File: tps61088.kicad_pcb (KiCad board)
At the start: 2 copper layers, 102 x 101.8 mm, 114 parts, among them J10 Conn_01x04, J11 Conn_01x04, J12 Conn_01x04, J13 Conn_01x04, J14 Conn_01x04, J2 Conn_01x12, J3 Conn_01x08, J5 Conn_01x02, J6 Conn_01x02, J7 Conn_01x04, J8 Conn_01x04, J9 Conn_01x04, P1 USB_C_Plug_USB2.0, SW1 SW_SPDT, SW2 SW_SPDT, SW3 SW_SPDT, SW4 SW_SPDT, SW5 SW_SPDT, SW6 SW_SPDT, SW7 SW_SPDT, U1 tps61088, U2 TPS5430DDA, U3 TPS5430DDA, U4 TPS5430DDA, U5 TPS5430DDA

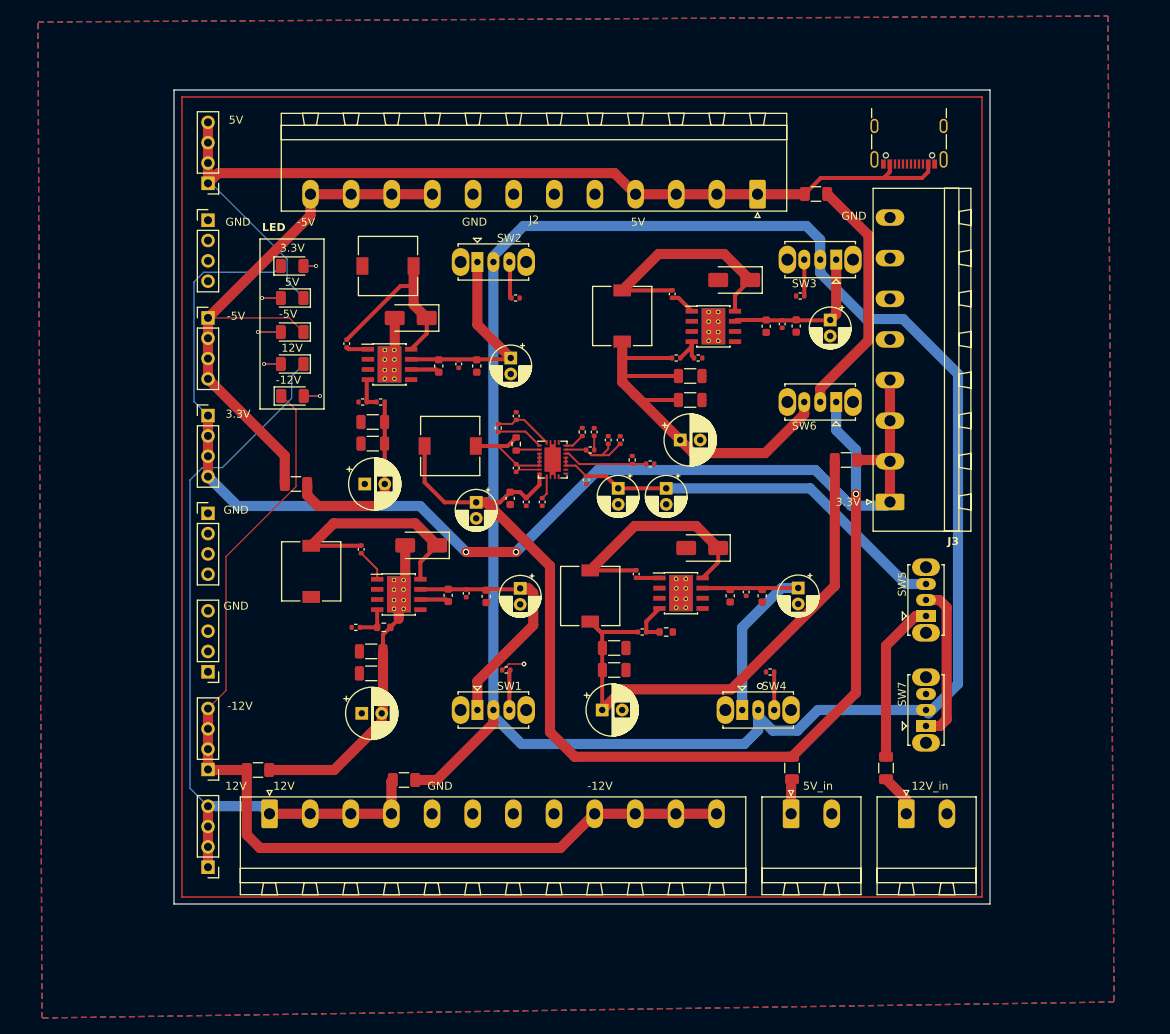
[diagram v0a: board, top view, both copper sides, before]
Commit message: V1.0
第一次下单PCB文件
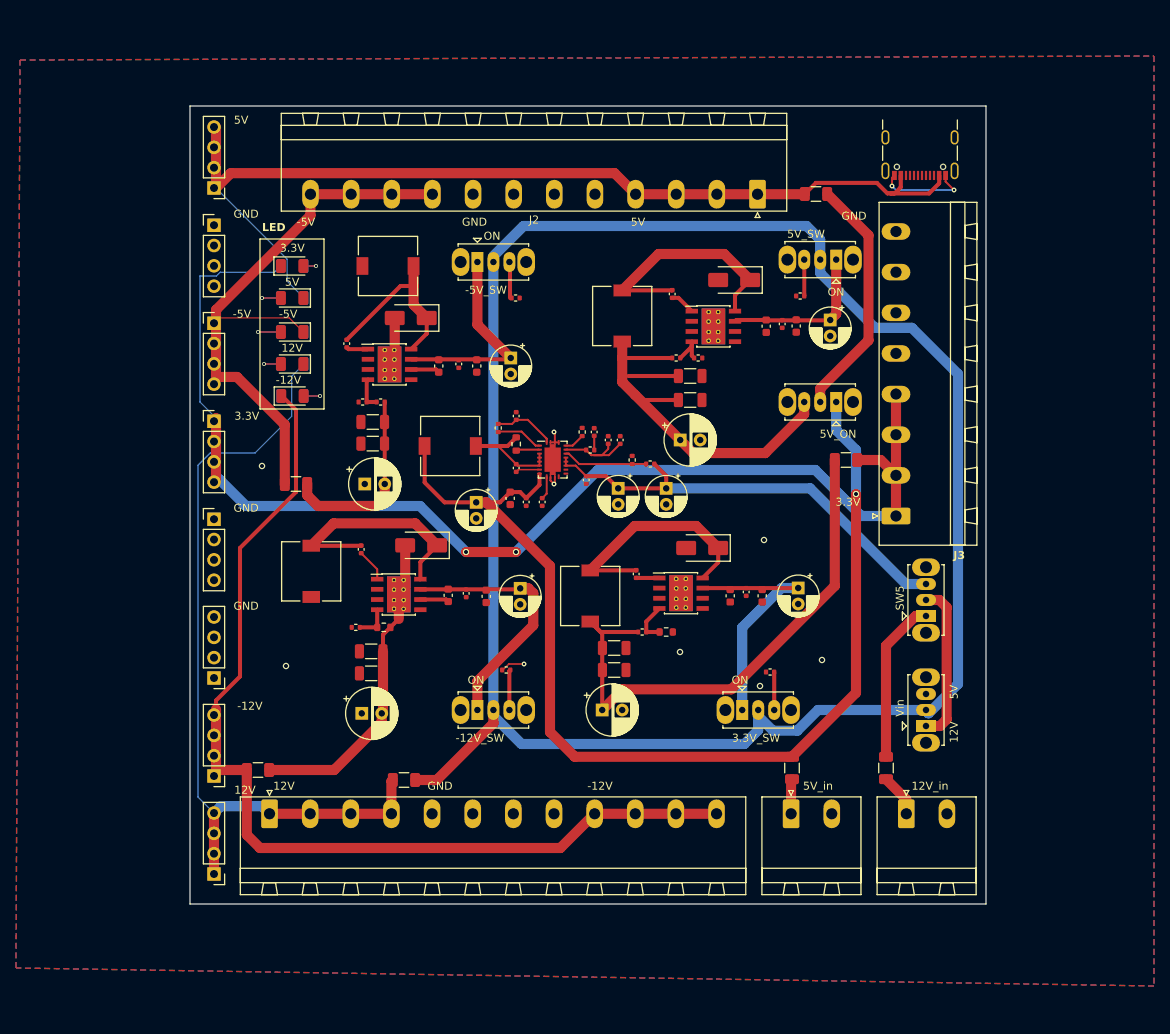
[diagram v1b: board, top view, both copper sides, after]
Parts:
- moved P1 1.98 mm to (191.5, 53.0)
- moved J3 1.90 mm to (188.5, 99.2)
- moved J7 1.14 mm to (103.2, 144.0)
- moved J8 1.11 mm to (103.2, 131.8)
- moved J14 1.08 mm to (103.2, 119.5)
- moved J13 1.05 mm to (103.2, 99.7)
- moved J12 1.03 mm to (103.2, 87.4)
- moved J11 1.00 mm to (103.2, 75.2)
- moved J10 0.97 mm to (103.2, 62.9)
- moved J9 0.95 mm to (103.2, 58.2)
- renumbered SW2 to -5V_SW, SW3 to 5V_SW, SW7 to Vin
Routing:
- net GND: track 3.05 -> 19.1 mm, vias 2 -> 11
- net Net-(SW5-C): track 52.1 -> 55.8 mm
- net Net-(J1-Pin_1): track 98.8 -> 100.6 mm
- net Net-(J12-Pin_1): track 151.6 -> 153.1 mm
- net Net-(D4-K): track 126.2 -> 124.8 mm
- net /5V_fuse: track 123.0 -> 123.9 mm
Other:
- board size 102 x 101.8 mm -> 99.5 x 99.8 mm
- board text added: "-12V_SW"
- board text added: "3.3V_SW"
- board text added: "5V_ON"
- board text added: "ON"
